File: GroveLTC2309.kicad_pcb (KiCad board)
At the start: 2 copper layers, 49.5 x 39.1 mm, 51 parts, among them P1 CONN_4_GROVE, P2 CONN_4_GROVE, P3 CONN_4_GROVE, P4 CONN_4_GROVE, P5 CONN_4_GROVE, P6 CONN_4_GROVE, P7 CONN_4_GROVE, P8 CONN_4_GROVE, P9 CONN_4_GROVE, U1 LM324, U2 LTC2309, U3 LM324

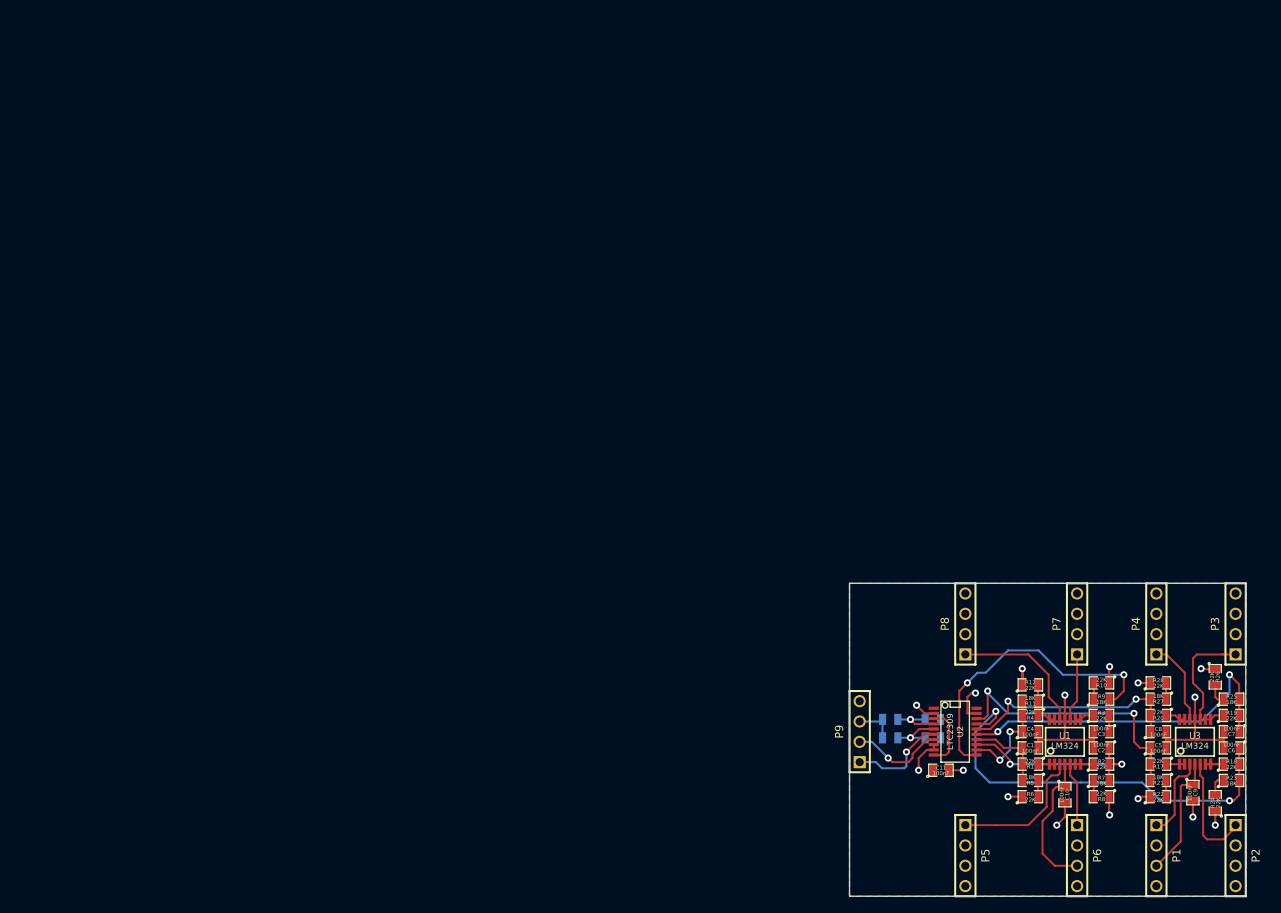
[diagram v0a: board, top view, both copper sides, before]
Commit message: version change to 2, first trial for layout revue
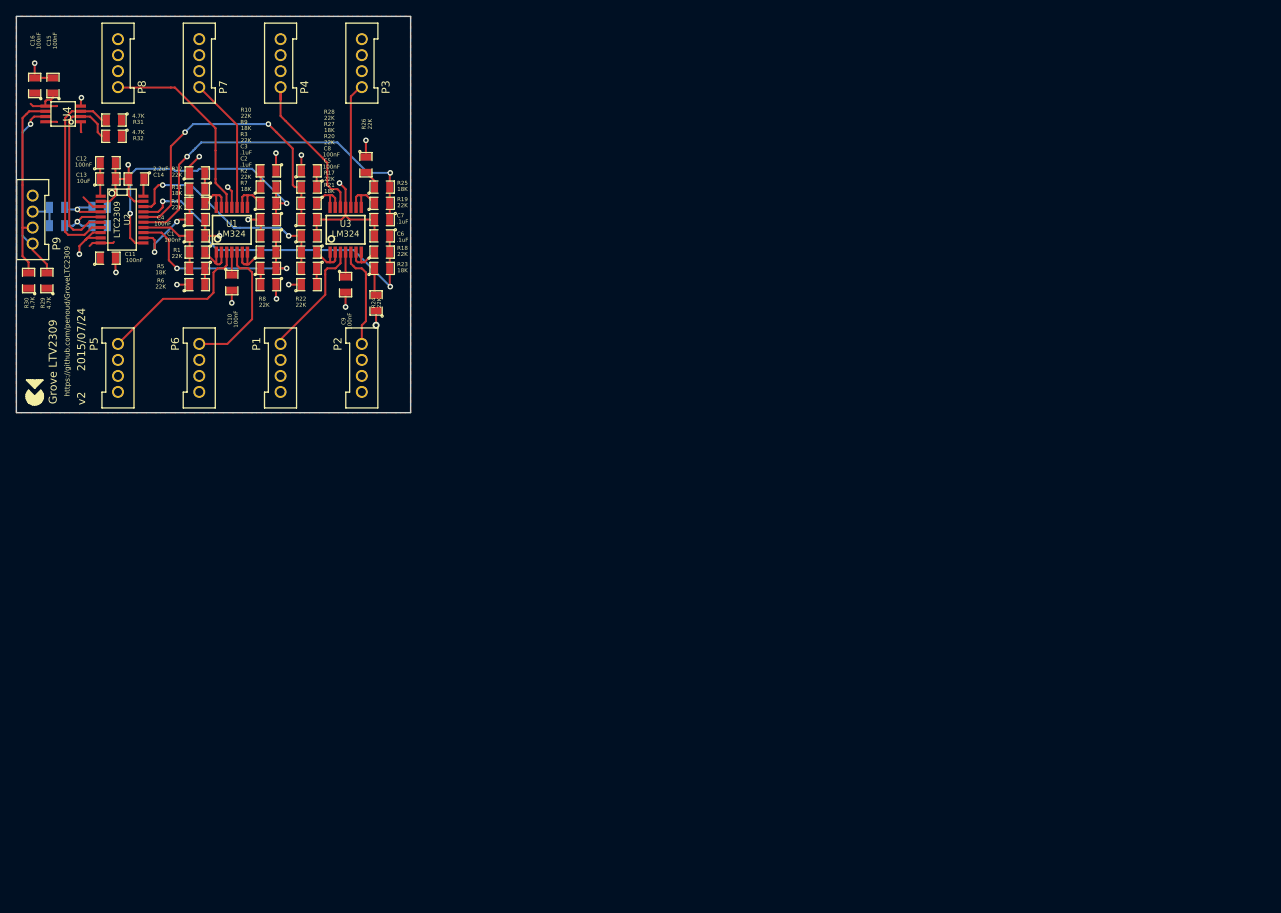
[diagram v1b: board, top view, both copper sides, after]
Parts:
- added C12: 100nF, SM0805, F.Cu at (120.7, 81.5)
- added C13: 10uF, SM0805, F.Cu at (120.7, 83.6)
- added C14: 2.2uF, SM0805, F.Cu at (124.2, 83.6)
- added C15: 100nF, SM0805, F.Cu at (113.8, 71.9)
- added C16: 100nF, SM0805, F.Cu at (111.5, 71.9)
- added R29: 4.7K, SM0805, F.Cu at (113.0, 96.3)
- added R30: 4.7K, SM0805, F.Cu at (110.7, 96.3)
- added R31: 4.7K, SM0805, F.Cu at (121.4, 76.2)
- added R32: 4.7K, SM0805, F.Cu at (121.4, 78.2)
- added U4: TCA9517A, SSOP8, F.Cu at (115.1, 75.4)
- C2, C3, C6, C7: value 100nF -> .1uF
- P1, P2, P3, P4, P5, P6, P7, P8, P9: footprint PIN_ARRAY_4x1 -> GROVE
- moved P7 130.2 mm to (132.1, 69.1)
- moved P4 130.0 mm to (142.2, 69.1)
- moved P3 129.8 mm to (152.4, 69.1)
- moved P8 127.0 mm to (121.9, 69.1)
- moved P6 125.5 mm to (132.1, 107.2)
- moved P1 125.3 mm to (142.2, 107.2)
- moved P2 125.1 mm to (152.4, 107.2)
- moved C6 124.0 mm to (154.9, 90.7)
- moved C7 124.0 mm to (154.9, 88.6)
- moved R18 124.0 mm to (154.9, 92.7)
- moved R19 124.0 mm to (154.9, 86.6)
- moved R23 124.0 mm to (154.9, 94.7)
- moved R25 124.0 mm to (154.9, 84.6)
- moved U3 124.0 mm to (150.4, 89.9)
- moved C5 124.0 mm to (145.8, 90.7)
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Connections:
- P9 pad 1: /ADC/SCL -> /TCA9517A/SCL_B
- P9 pad 2: /ADC/SDA -> /TCA9517A/SDA_B
- U2 pad 1: (no net) -> N-0000042
- U2 pad 20: (no net) -> N-0000041
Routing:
- net /TCA9517A/SDA_B: track 0.00 -> 24.2 mm
- net /TCA9517A/SCL_B: track 0.00 -> 23.0 mm, vias 0 -> 1
- net +5V: track 46.5 -> 25.0 mm
- net /ADC/SDA: track 11.8 -> 25.1 mm, vias 1 -> 0
- net /ADC/SCL: track 12.4 -> 24.2 mm, vias 1 -> 0
- net /ADC/CH2: track 28.8 -> 38.9 mm
- net /Amplifier2/IN1: track 7.98 -> 17.6 mm
- net /Amplifier1/IN3: track 10.6 -> 20.2 mm
- net /ADC/CH1: track 52.5 -> 43.5 mm
- net /Amplifier2/IN2: track 8.49 -> 17.0 mm
- net /ADC/CH0: track 36.6 -> 28.6 mm
- net /Amplifier2/IN3: track 17.6 -> 24.8 mm
- net /Amplifier1/IN0: track 10.5 -> 15.4 mm
- net /ADC/CH7: track 42.1 -> 37.8 mm
- net N-0000042: track 0.00 -> 4.22 mm
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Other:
- board size 49.5 x 39.1 mm -> 49.3 x 49.5 mm
- net class Default: via_dia 0.889 -> 0.7; via_drill 0.635 -> 0.5
- rule via_min_drill: 0.508 -> 0.5
- rule via_min_size: 0.889 -> 0.7
- board text added: "2015/07/24"
- board text added: "Grove LTV2309"
- board text added: "https://github.com/penoud/GroveLTC2309"
- board text added: "v2"
